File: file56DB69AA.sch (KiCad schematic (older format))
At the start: 1 part, among them U3 MPU-9250

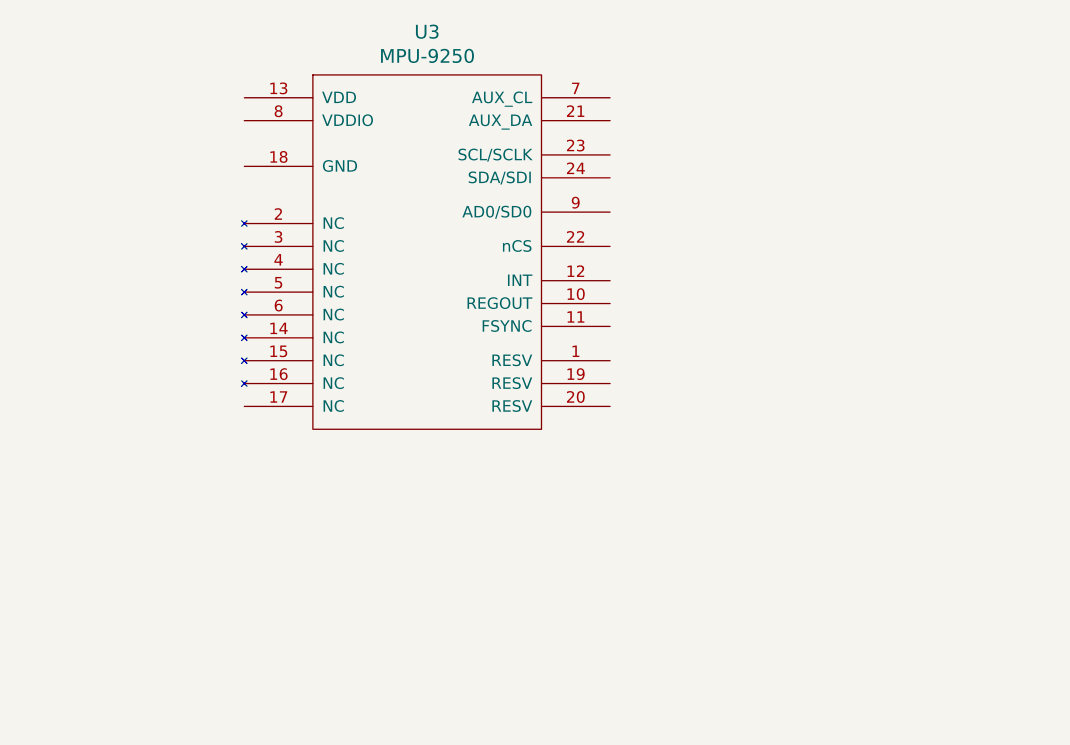
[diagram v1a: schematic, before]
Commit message: started layout, completed schematic
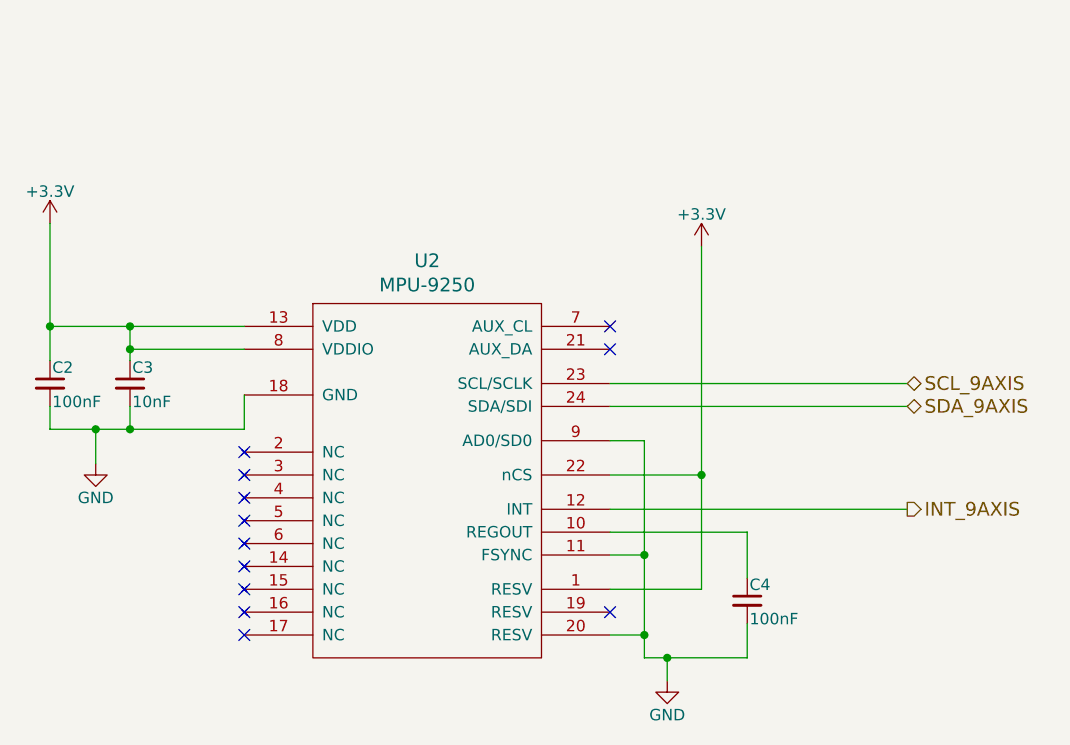
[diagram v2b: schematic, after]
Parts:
- added C2, C4: 100nF, symbol C_Small
- added C3: 10nF, symbol C_Small
- renumbered U3 to U2
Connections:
- net +3V3: now reaches U2.1 (RESV)
- net +3V3: now also U2.13 (VDD), U2.22 (nCS), U2.8 (VDDIO), C2.1, C3.1
- net at U2.10 (REGOUT): now also C4.1
- net GND: now reaches U2.11 (FSYNC)
- net GND: now also U2.18 (GND), U2.20 (RESV), U2.9 (AD0/SD0), C2.2, C3.2, C4.2
- net INT_9AXIS: now reaches U2.12 (INT)
- net SCL_9AXIS: now reaches U2.23 (SCL/SCLK)
- net SDA_9AXIS: now reaches U2.24 (SDA/SDI)
- no-connect marks 0 -> 12
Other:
- moved on the sheet: U2
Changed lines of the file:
@@
 LIBS:mpu-9250
 LIBS:SAMD21E17A
+LIBS:miniultrapro
+LIBS:texas-instruments
 LIBS:lorawan_gps-cache
 EELAYER 25 0
@@
 $Descr A4 11693 8268
 encoding utf-8
-Sheet 4 7
+Sheet 3 7
 Title ""
 Date ""
@@
 $EndDescr
 $Comp
-L MPU-9250 U3
+L MPU-9250 U2
 U 1 1 56DB6A06
-P 5650 3400
-F 0 "U3" H 5650 4337 60  0000 C CNN
-F 1 "MPU-9250" H 5650 4231 60  0000 C CNN
-F 2 "mpu-9250:MPU-9250" H 5650 4000 60  0001 C CNN
-F 3 "" H 5650 4000 60  0000 C CNN
-	1    5650 3400
+P 5650 4400
+F 0 "U2" H 5650 5337 60  0000 C CNN
+F 1 "MPU-9250" H 5650 5231 60  0000 C CNN
+F 2 "mpu-9250:MPU-9250" H 5650 5000 60  0001 C CNN
+F 3 "" H 5650 5000 60  0000 C CNN
+	1    5650 4400
 	1    0    0    -1
 $EndComp
+NoConn ~ 4850 4300
+NoConn ~ 4850 4400
+NoConn ~ 4850 4500
+NoConn ~ 4850 4600
+NoConn ~ 4850 4700
+NoConn ~ 4850 4800
+NoConn ~ 4850 4900
+NoConn ~ 4850 5000
+NoConn ~ 4850 5100
+$Comp
+L C_Small C2
+U 1 1 56EA6CE4
+P 4000 4000
+F 0 "C2" H 4010 4070 50  0000 L CNN
+F 1 "100nF" H 4010 3920 50  0000 L CNN
+F 2 "" H 4000 4000 50  0000 C CNN
+F 3 "" H 4000 4000 50  0000 C CNN
+	1    4000 4000
+	1    0    0    -1
+$EndComp
+$Comp
+L C_Small C3
+U 1 1 56EA6D67
+P 4350 4000
+F 0 "C3" H 4360 4070 50  0000 L CNN
+F 1 "10nF" H 4360 3920 50  0000 L CNN
+F 2 "" H 4350 4000 50  0000 C CNN
+F 3 "" H 4350 4000 50  0000 C CNN
+	1    4350 4000
+	1    0    0    -1
+$EndComp
+Text HLabel 7750 4100 2    60   BiDi ~ 0
+SDA_9AXIS
+Text HLabel 7750 4000 2    60   BiDi ~ 0
+SCL_9AXIS
+$Comp
+L GND #PWR5
+U 1 1 56EA6F16
+P 4200 4350
+F 0 "#PWR5" H 4200 4100 50  0001 C CNN
+F 1 "GND" H 4200 4200 50  0000 C CNN
+F 2 "" H 4200 4350 50  0000 C CNN
+F 3 "" H 4200 4350 50  0000 C CNN
+	1    4200 4350
+	1    0    0    -1
+$EndComp
+$Comp
+L GND #PWR6
+U 1 1 56EA6F51
+P 6700 5300
+F 0 "#PWR6" H 6700 5050 50  0001 C CNN
+F 1 "GND" H 6700 5150 50  0000 C CNN
+F 2 "" H 6700 5300 50  0000 C CNN
+F 3 "" H 6700 5300 50  0000 C CNN
+	1    6700 5300
+	1    0    0    -1
+$EndComp
+$Comp
+L +3.3V #PWR4
+U 1 1 56EA6F6B
+P 4000 3300
+F 0 "#PWR4" H 4000 3150 50  0001 C CNN
+F 1 "+3.3V" H 4000 3440 50  0000 C CNN
+F 2 "" H 4000 3300 50  0000 C CNN
+F 3 "" H 4000 3300 50  0000 C CNN
+	1    4000 3300
+	1    0    0    -1
+$EndComp
+NoConn ~ 6450 3750
+NoConn ~ 6450 3850
+$Comp
+L +3.3V #PWR7
+U 1 1 56EA7925
+P 6850 3400
+F 0 "#PWR7" H 6850 3250 50  0001 C CNN
+F 1 "+3.3V" H 6850 3540 50  0000 C CNN
+F 2 "" H 6850 3400 50  0000 C CNN
+F 3 "" H 6850 3400 50  0000 C CNN
+	1    6850 3400
+	1    0    0    -1
+$EndComp
+$Comp
+L C_Small C4
+U 1 1 56EA7A89
+P 7050 4950
+F 0 "C4" H 7060 5020 50  0000 L CNN
+F 1 "100nF" H 7060 4870 50  0000 L CNN
+F 2 "" H 7050 4950 50  0000 C CNN
+F 3 "" H 7050 4950 50  0000 C CNN
+	1    7050 4950
+	1    0    0    -1
+$EndComp
+Text HLabel 7750 4550 2    60   Output ~ 0
+INT_9AXIS
+NoConn ~ 6450 5000
+Wire Wire Line
+	4000 3750 4850 3750
+Wire Wire Line
+	4000 3300 4000 3900
+Wire Wire Line
+	4850 3850 4350 3850
+Wire Wire Line
+	4350 3750 4350 3900
+Connection ~ 4000 3750
+Connection ~ 4350 3750
+Connection ~ 4350 3850
+Wire Wire Line
+	4850 4200 4850 4050
+Wire Wire Line
+	4000 4200 4850 4200
+Wire Wire Line
+	4350 4100 4350 4200
+Connection ~ 4350 4200
+Wire Wire Line
+	4200 4350 4200 4200
+Connection ~ 4200 4200
+Wire Wire Line
+	7050 4650 7050 4850
+Wire Wire Line
+	6450 4750 6600 4750
+Wire Wire Line
+	6600 4250 6600 5200
+Wire Wire Line
+	6600 5200 7050 5200
+Wire Wire Line
+	6700 5200 6700 5300
+Connection ~ 6700 5200
+Wire Wire Line
+	6450 4250 6600 4250
+Connection ~ 6600 4750
+Wire Wire Line
+	4000 4200 4000 4100
+Wire Wire Line
+	6450 5100 6600 5100
+Connection ~ 6600 5100
+Wire Wire Line
+	6450 4650 7050 4650
+Wire Wire Line
+	7050 5200 7050 5050
+Wire Wire Line
+	6450 4900 6850 4900
+Wire Wire Line
+	6850 4900 6850 3400
+Wire Wire Line
+	6450 4400 6850 4400
+Connection ~ 6850 4400
+Wire Wire Line
+	6450 4550 7750 4550
+Wire Wire Line
+	6450 4100 7750 4100
+Wire Wire Line
+	6450 4000 7750 4000
 $EndSCHEMATC
